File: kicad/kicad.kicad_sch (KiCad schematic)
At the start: 256 parts, among them J1 USB_B_Micro, J2 SWD, J3 pwr_led+, J4 pwr_led-, J5 caps_led+, J6 caps_led-, U1 AMS1117-3.3, Y1 16MGz, sw1 Esc, sw10 Z, sw100 N5, sw101 N6, sw102 N2, sw103 N1, sw104 N0, sw105 MPlay, sw106 MFwd, sw107 NSlash, sw108 NStar, sw109 N8, sw11 LCtrl, sw110 N9, sw111 NMinus, sw112 NPlus, sw113 NEnter, sw114 N3, sw115 NPeriod, sw12 LSys, sw13 F2, sw14 F3, sw15 2, sw16 3, sw17 W, sw18 E, sw19 S, sw2 F1, sw20 D, sw21 X, sw22 C, sw23 LAlt, sw24 THome, sw25 F4, sw26 F5, sw27 4, sw28 5, sw29 R, sw3 Tilda, sw30 T, sw31 F, sw32 G, sw33 V, sw34 B, sw35 LSpace, sw36 TLeft, sw37 F6, sw38 F7, sw39 6, sw4 1, sw40 7, sw41 Y, sw42 U, sw43 H, sw44 J, sw45 N, sw46 M, sw47 TUp, sw48 TDown, sw49 F8, sw5 Tab, sw50 F9, sw51 8, sw52 9, sw53 I, sw54 O, sw55 K, sw56 L, sw57 Comma, sw58 Period, sw59 RSpace, sw6 Q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

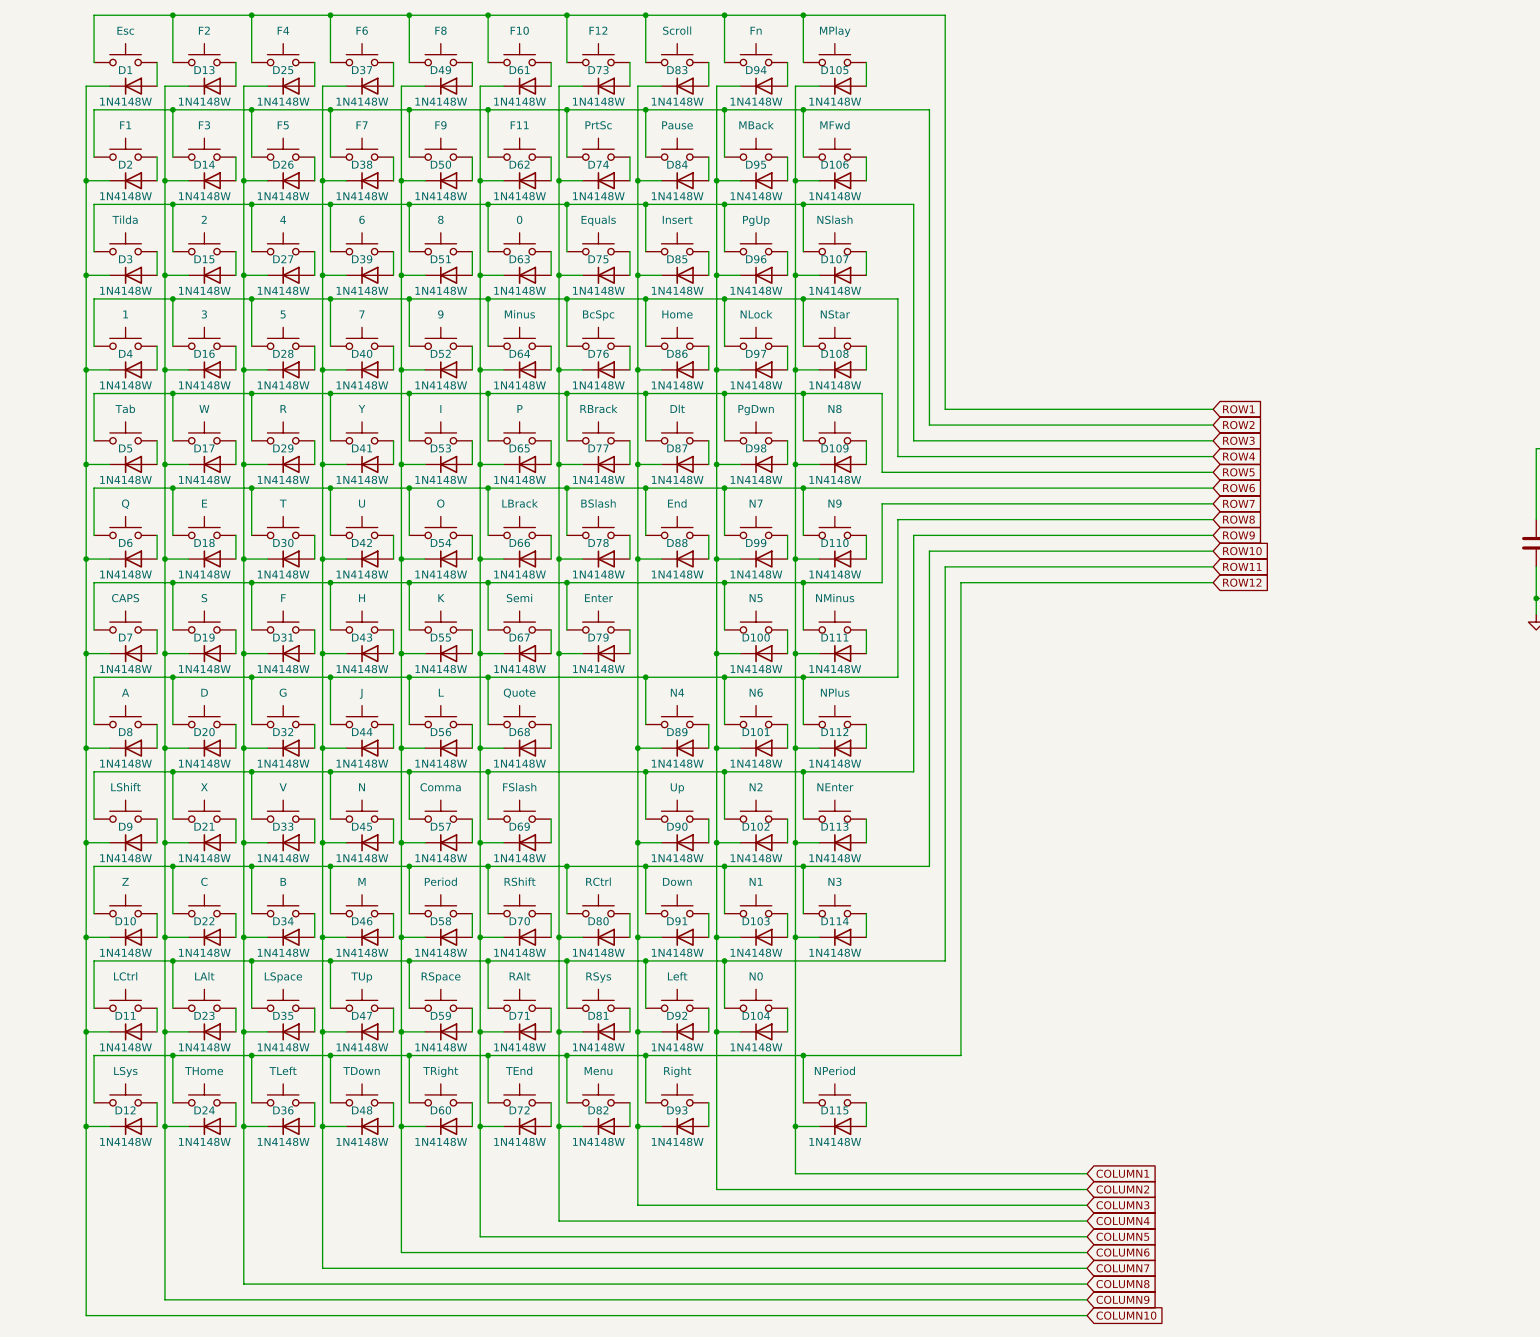
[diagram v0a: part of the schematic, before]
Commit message: 75% layout
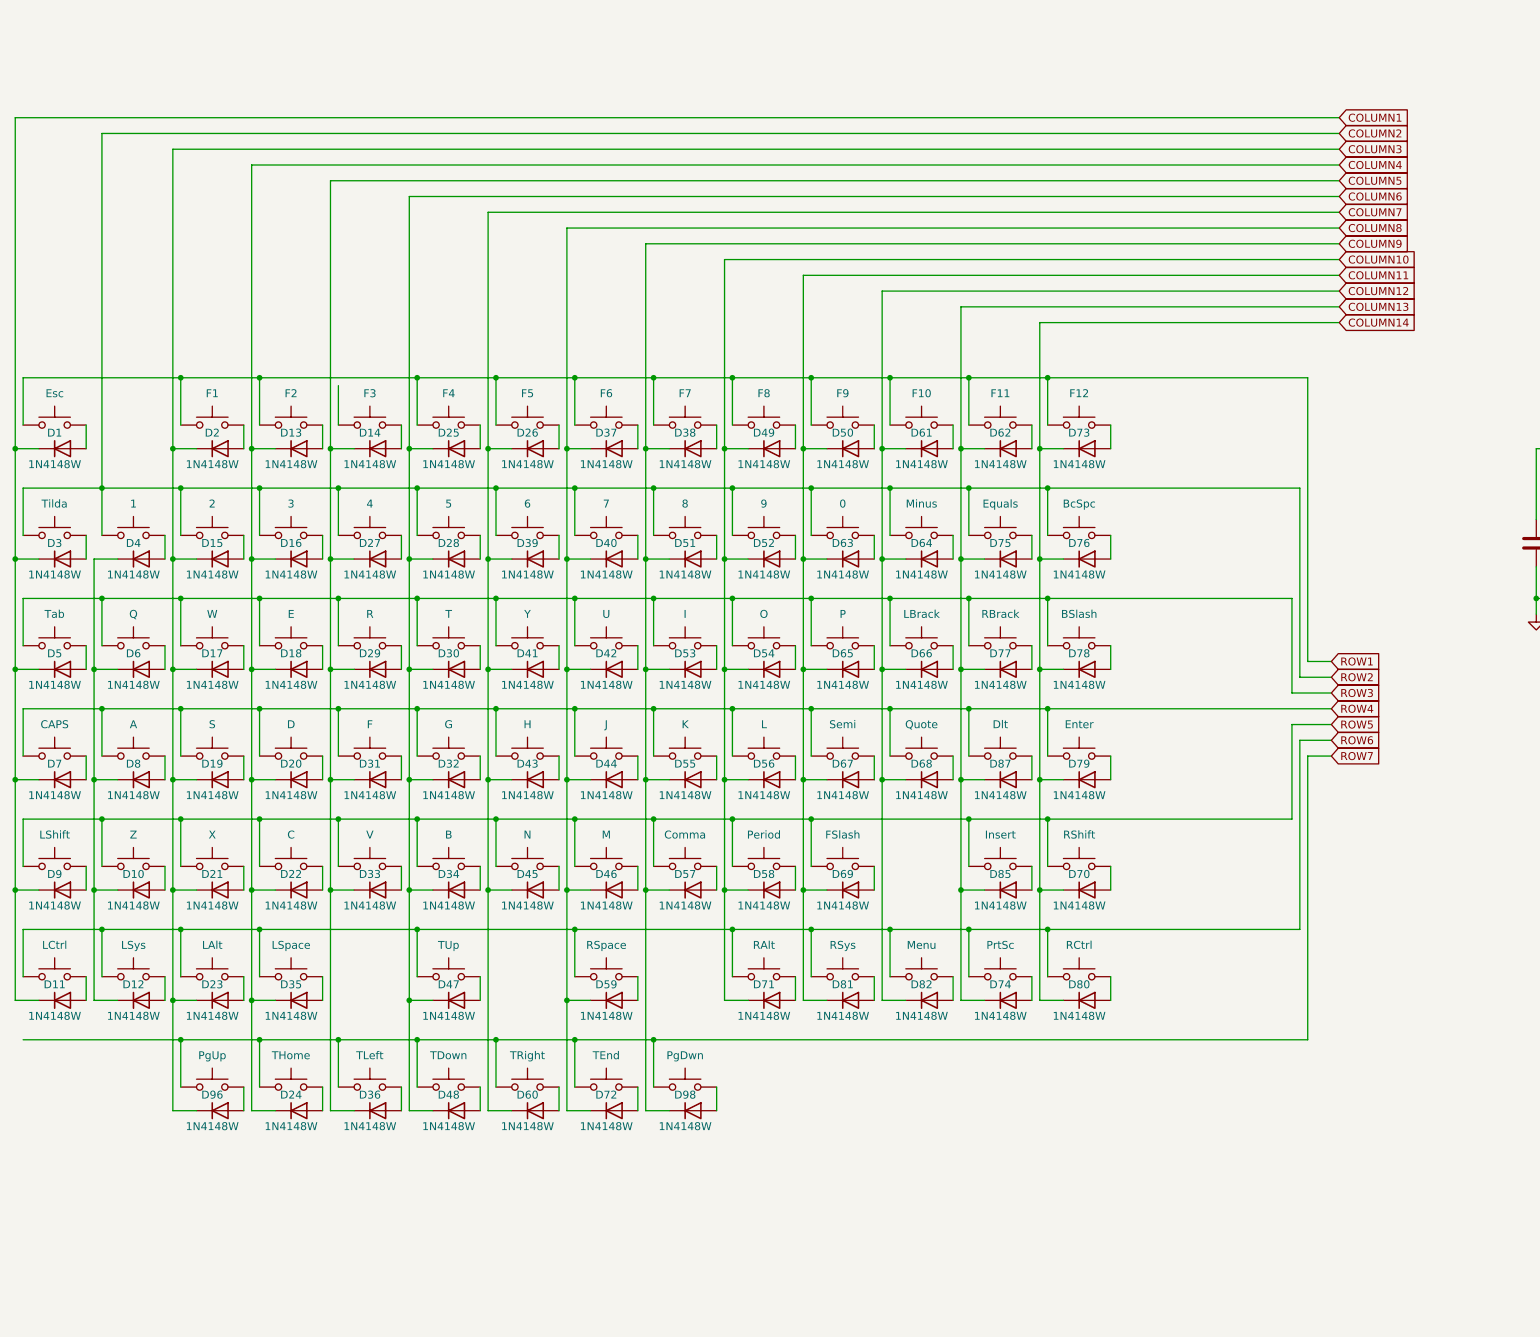
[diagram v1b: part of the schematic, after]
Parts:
- removed D100, D101, D102, D103, D104, D105, D106, D107, D108, D109, D110, D111, D112, D113, D114, D115, D83, D84, D86, D88, D89, D90, D91, D92, D93, D94, D95, D97, D99: 1N4148W, Diode_SMD:D_SOD-123, symbol Diode:1N4148W
- removed sw100: N5, Button_Switch_Keyboard:SW_Cherry_MX_1.00u_PCB, symbol Switch:SW_Push
- removed sw101: N6, Button_Switch_Keyboard:SW_Cherry_MX_1.00u_PCB, symbol Switch:SW_Push
- removed sw102: N2, Button_Switch_Keyboard:SW_Cherry_MX_1.00u_PCB, symbol Switch:SW_Push
- removed sw103: N1, Button_Switch_Keyboard:SW_Cherry_MX_1.00u_PCB, symbol Switch:SW_Push
- removed sw104: N0, Button_Switch_Keyboard:SW_Cherry_MX_2.00u_PCB, symbol Switch:SW_Push
- removed sw105: MPlay, Button_Switch_Keyboard:SW_Cherry_MX_1.00u_PCB, symbol Switch:SW_Push
- removed sw106: MFwd, Button_Switch_Keyboard:SW_Cherry_MX_1.00u_PCB, symbol Switch:SW_Push
- removed sw107: NSlash, Button_Switch_Keyboard:SW_Cherry_MX_1.00u_PCB, symbol Switch:SW_Push
- removed sw108: NStar, Button_Switch_Keyboard:SW_Cherry_MX_1.00u_PCB, symbol Switch:SW_Push
- removed sw109: N8, Button_Switch_Keyboard:SW_Cherry_MX_1.00u_PCB, symbol Switch:SW_Push
- removed sw110: N9, Button_Switch_Keyboard:SW_Cherry_MX_1.00u_PCB, symbol Switch:SW_Push
- removed sw111: NMinus, Button_Switch_Keyboard:SW_Cherry_MX_1.00u_PCB, symbol Switch:SW_Push
- removed sw112: NPlus, Button_Switch_Keyboard:SW_Cherry_MX_2.00u_Vertical_PCB, symbol Switch:SW_Push
- removed sw113: NEnter, Button_Switch_Keyboard:SW_Cherry_MX_2.00u_Vertical_PCB, symbol Switch:SW_Push
- removed sw114: N3, Button_Switch_Keyboard:SW_Cherry_MX_1.00u_PCB, symbol Switch:SW_Push
- removed sw115: NPeriod, Button_Switch_Keyboard:SW_Cherry_MX_1.00u_PCB, symbol Switch:SW_Push
- removed sw83: Scroll, Button_Switch_Keyboard:SW_Cherry_MX_1.00u_PCB, symbol Switch:SW_Push
- removed sw84: Pause, Button_Switch_Keyboard:SW_Cherry_MX_1.00u_PCB, symbol Switch:SW_Push
- removed sw86: Home, Button_Switch_Keyboard:SW_Cherry_MX_1.00u_PCB, symbol Switch:SW_Push
- removed sw88: End, Button_Switch_Keyboard:SW_Cherry_MX_1.00u_PCB, symbol Switch:SW_Push
- removed sw89: N4, Button_Switch_Keyboard:SW_Cherry_MX_1.00u_PCB, symbol Switch:SW_Push
- removed sw90: Up, Button_Switch_Keyboard:SW_Cherry_MX_1.00u_PCB, symbol Switch:SW_Push
- removed sw91: Down, Button_Switch_Keyboard:SW_Cherry_MX_1.00u_PCB, symbol Switch:SW_Push
- removed sw92: Left, Button_Switch_Keyboard:SW_Cherry_MX_1.00u_PCB, symbol Switch:SW_Push
- removed sw93: Right, Button_Switch_Keyboard:SW_Cherry_MX_1.00u_PCB, symbol Switch:SW_Push
- removed sw94: Fn, Button_Switch_Keyboard:SW_Cherry_MX_1.00u_PCB, symbol Switch:SW_Push
- removed sw95: MBack, Button_Switch_Keyboard:SW_Cherry_MX_1.00u_PCB, symbol Switch:SW_Push
- removed sw97: NLock, Button_Switch_Keyboard:SW_Cherry_MX_1.00u_PCB, symbol Switch:SW_Push
- removed sw99: N7, Button_Switch_Keyboard:SW_Cherry_MX_1.00u_PCB, symbol Switch:SW_Push
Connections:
- net COLUMN1: now also D1.1 (K), D11.1 (K), D3.1 (K), D5.1 (K), D7.1 (K), D9.1 (K)
- net COLUMN10: now also D49.1 (K), D52.1 (K), D54.1 (K), D56.1 (K), D58.1 (K), D71.1 (K); no longer D1.1 (K), D10.1 (K), D11.1 (K), D12.1 (K), D2.1 (K), D3.1 (K), D4.1 (K), D5.1 (K), D6.1 (K), D7.1 (K), D8.1 (K), D9.1 (K)
- net COLUMN2: now also MCU1.39 (PC8), sw15.1, sw16.1, sw27.1, sw28.1, sw3.1, sw39.1, sw4.1, sw40.1, sw51.1, sw52.1, sw63.1, sw64.1, sw75.1, sw76.1; no longer D96.1 (K), D98.1 (K)
- net COLUMN3: now also D15.1 (K), D17.1 (K), D19.1 (K), D2.1 (K), D21.1 (K), D23.1 (K), D96.1 (K); no longer D85.1 (K), D87.1 (K)
- net COLUMN4: now also D13.1 (K), D16.1 (K), D18.1 (K), D20.1 (K), D22.1 (K), D24.1 (K), D35.1 (K); no longer D73.1 (K), D74.1 (K), D75.1 (K), D76.1 (K), D77.1 (K), D78.1 (K), D79.1 (K), D80.1 (K), D81.1 (K), D82.1 (K)
- net COLUMN5: now also D14.1 (K), D27.1 (K), D29.1 (K), D31.1 (K), D33.1 (K), D36.1 (K); no longer D61.1 (K), D62.1 (K), D63.1 (K), D64.1 (K), D65.1 (K), D66.1 (K), D67.1 (K), D68.1 (K), D69.1 (K), D70.1 (K), D71.1 (K), D72.1 (K)
- net COLUMN6: now also D25.1 (K), D28.1 (K), D30.1 (K), D32.1 (K), D34.1 (K), D47.1 (K), D48.1 (K); no longer D49.1 (K), D50.1 (K), D51.1 (K), D52.1 (K), D53.1 (K), D54.1 (K), D55.1 (K), D56.1 (K), D57.1 (K), D58.1 (K), D59.1 (K), D60.1 (K)
- net COLUMN7: now also D26.1 (K), D60.1 (K); no longer D37.1 (K), D38.1 (K), D40.1 (K), D42.1 (K), D44.1 (K), D46.1 (K), D47.1 (K), D48.1 (K)
- net COLUMN8: now also D37.1 (K), D40.1 (K), D42.1 (K), D44.1 (K), D46.1 (K), D59.1 (K), D72.1 (K); no longer D25.1 (K), D26.1 (K), D27.1 (K), D28.1 (K), D29.1 (K), D30.1 (K), D31.1 (K), D32.1 (K), D33.1 (K), D34.1 (K), D35.1 (K), D36.1 (K)
- net COLUMN9: now also D38.1 (K), D51.1 (K), D53.1 (K), D55.1 (K), D57.1 (K), D98.1 (K); no longer D13.1 (K), D14.1 (K), D15.1 (K), D16.1 (K), D17.1 (K), D18.1 (K), D19.1 (K), D20.1 (K), D21.1 (K), D22.1 (K), D23.1 (K), D24.1 (K)
- net ROW1: now also sw2.1, sw26.1, sw38.1, sw50.1, sw62.1
- net ROW10: no longer sw10.1, sw22.1, sw34.1, sw46.1, sw58.1, sw70.1, sw80.1
- net ROW11: no longer sw11.1, sw23.1, sw35.1, sw47.1, sw59.1, sw71.1, sw81.1
- net ROW12: no longer sw12.1, sw24.1, sw36.1, sw48.1, sw60.1, sw72.1, sw82.1
- net ROW3: now also sw17.1, sw18.1, sw29.1, sw30.1, sw41.1, sw42.1, sw5.1, sw53.1, sw54.1, sw6.1, sw65.1, sw66.1, sw77.1, sw78.1; no longer sw15.1, sw27.1, sw3.1, sw39.1, sw51.1, sw63.1, sw75.1, sw85.1, sw96.1
- net ROW4: now also sw19.1, sw20.1, sw31.1, sw32.1, sw43.1, sw44.1, sw55.1, sw56.1, sw67.1, sw68.1, sw7.1, sw79.1, sw8.1, sw87.1; no longer sw16.1, sw28.1, sw4.1, sw40.1, sw52.1, sw64.1, sw76.1
- net ROW5: now also sw10.1, sw21.1, sw22.1, sw33.1, sw34.1, sw45.1, sw46.1, sw57.1, sw58.1, sw69.1, sw70.1, sw85.1, sw9.1; no longer sw17.1, sw29.1, sw41.1, sw5.1, sw53.1, sw65.1, sw77.1, sw87.1, sw98.1
- net ROW6: now also sw11.1, sw12.1, sw23.1, sw35.1, sw47.1, sw59.1, sw71.1, sw74.1, sw80.1, sw81.1, sw82.1; no longer sw18.1, sw30.1, sw42.1, sw54.1, sw6.1, sw66.1, sw78.1
- net ROW7: now also sw24.1, sw36.1, sw48.1, sw60.1, sw72.1, sw96.1, sw98.1; no longer sw19.1, sw31.1, sw43.1, sw55.1, sw67.1, sw7.1, sw79.1
- net ROW8: no longer sw20.1, sw32.1, sw44.1, sw56.1, sw68.1, sw8.1
- net ROW9: no longer sw21.1, sw33.1, sw45.1, sw57.1, sw69.1, sw9.1
- removed net ROW2: MCU1.39 (PC8), sw14.1, sw2.1, sw26.1, sw38.1, sw50.1, sw62.1, sw74.1
- new net: D10.1 (K), D12.1 (K), D4.1 (K), D6.1 (K), D8.1 (K)
- new net COLUMN11: D50.1 (K), D63.1 (K), D65.1 (K), D67.1 (K), D69.1 (K), D81.1 (K)
- new net COLUMN12: D61.1 (K), D64.1 (K), D66.1 (K), D68.1 (K), D82.1 (K)
- new net COLUMN13: D62.1 (K), D74.1 (K), D75.1 (K), D77.1 (K), D85.1 (K), D87.1 (K)
- new net COLUMN14: D70.1 (K), D73.1 (K), D76.1 (K), D78.1 (K), D79.1 (K), D80.1 (K)
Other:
- moved on the sheet: D1, D10, D11, D12, D13, D14, D15, D16, D17, D18, D19, D2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
